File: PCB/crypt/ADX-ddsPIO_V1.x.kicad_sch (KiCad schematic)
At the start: 74 parts, among them J1 Conn_Coaxial, J2 +12V, Q1 BS170, Q2 BS170, Q3 BS170, Q5 BS170, U1 L7805, U2 74LS244, U4 CD2003GB_GP

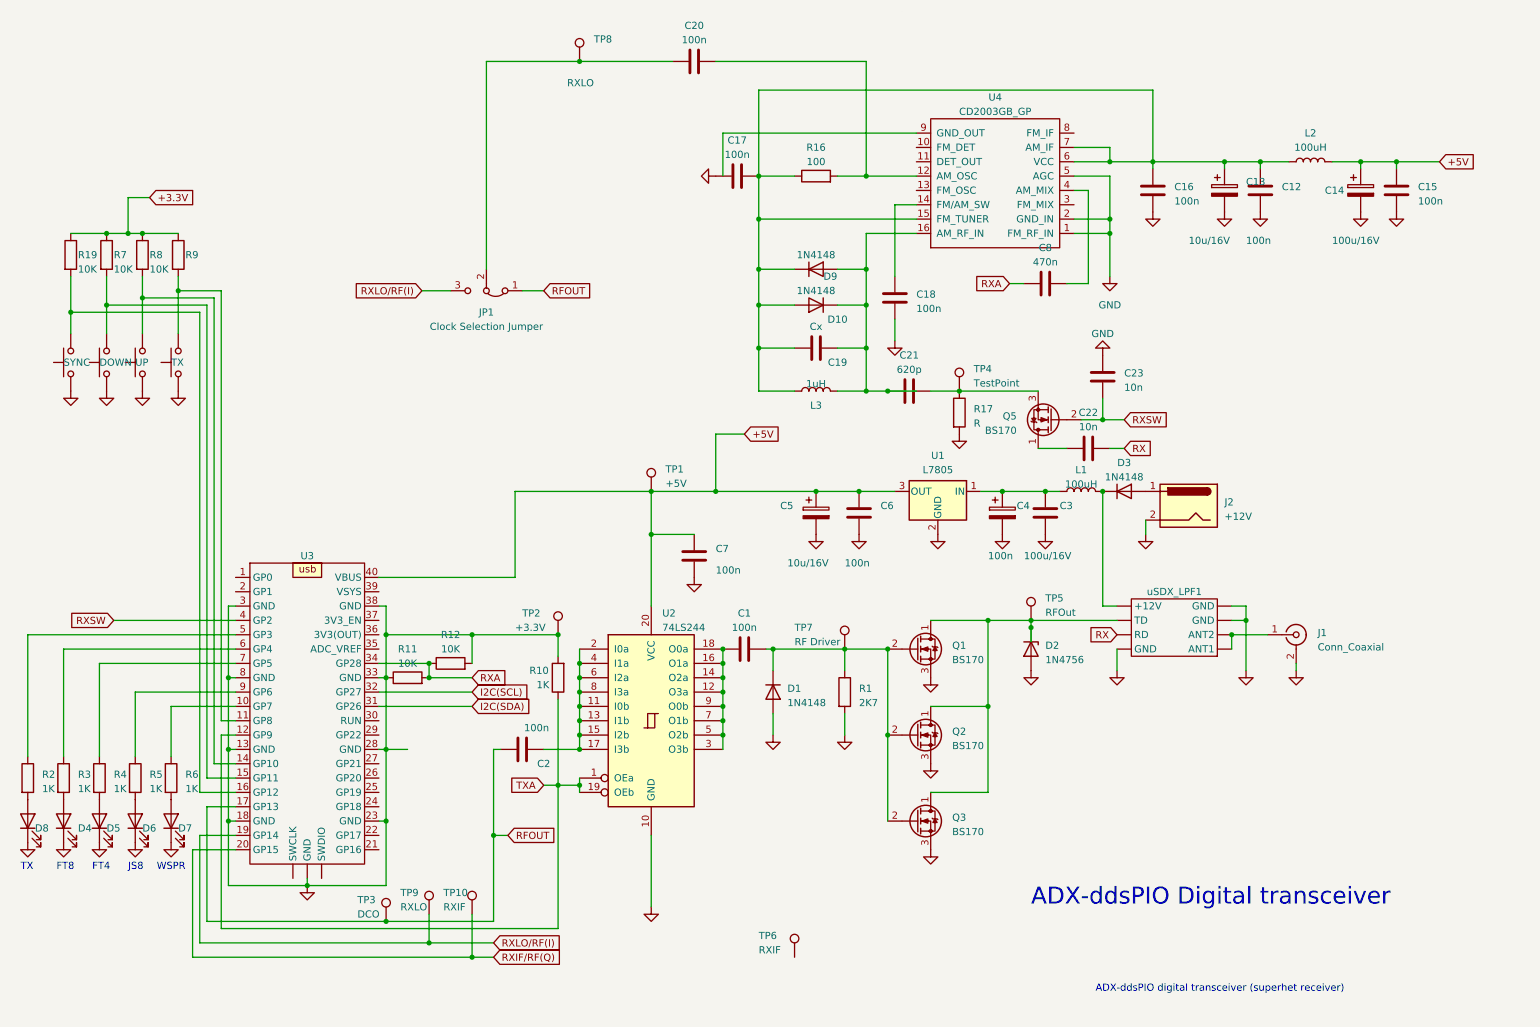
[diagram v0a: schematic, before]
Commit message: wiring
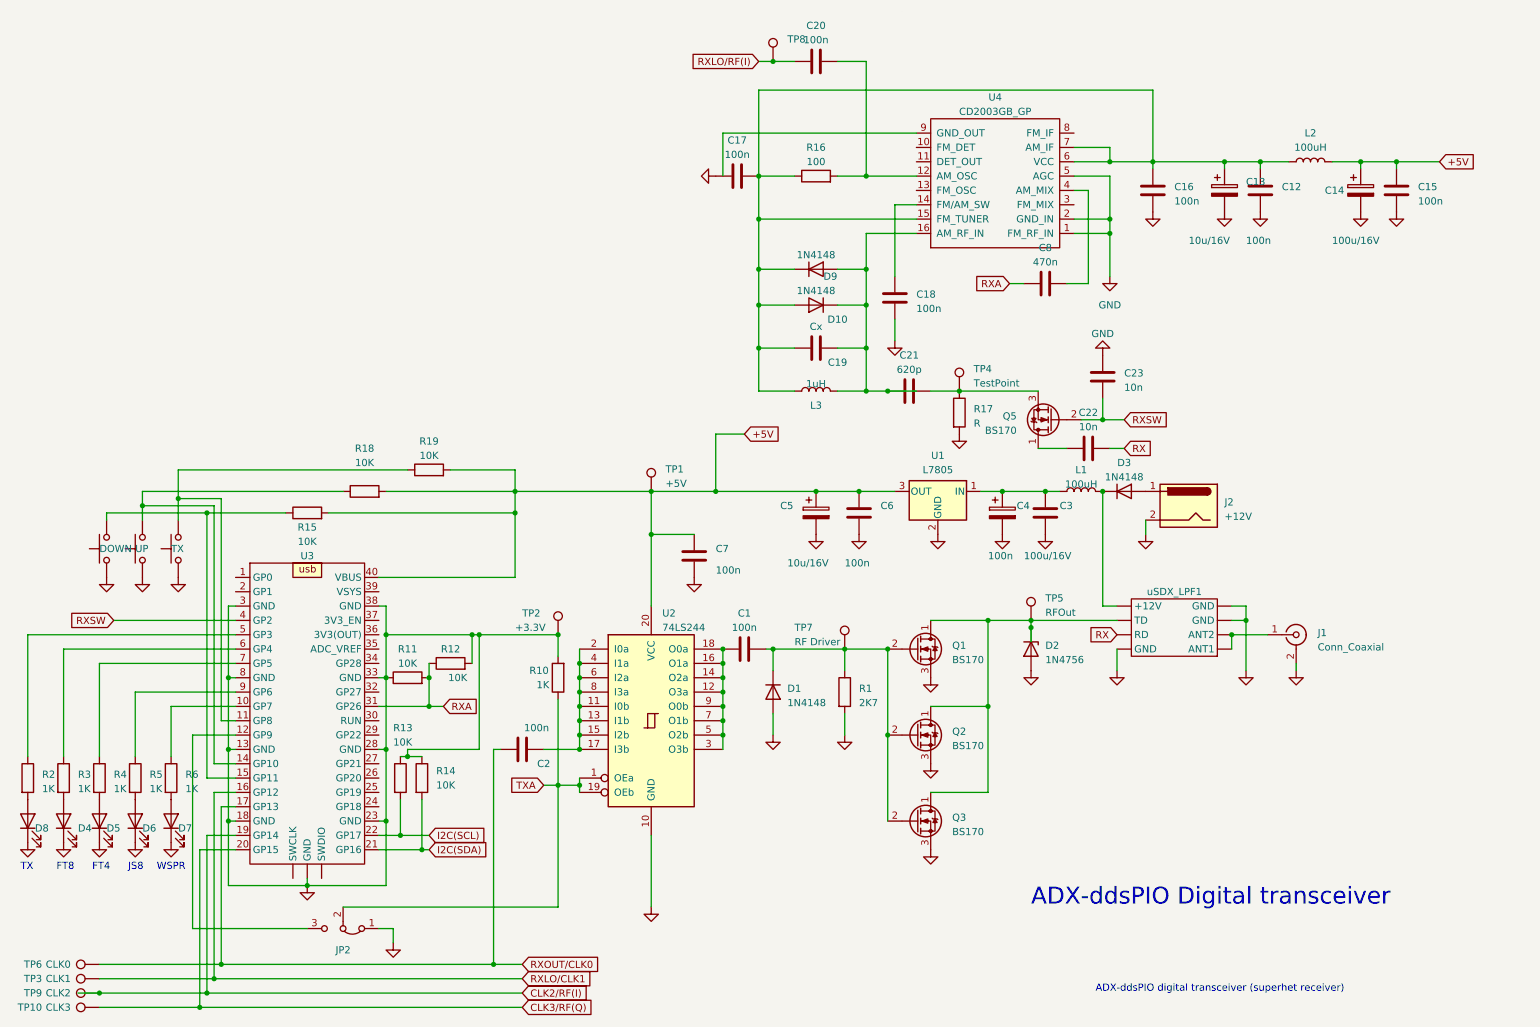
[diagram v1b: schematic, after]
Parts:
- removed JP1: Clock Selection Jumper, symbol Jumper:Jumper_3_Bridged12
- removed R7, R8, R9: 10K, symbol Device:R
- removed SYNC: SW_MEC_5G, symbol Switch:SW_MEC_5G
- added JP2: ~, symbol Jumper:Jumper_3_Bridged12
- added R13, R14, R15, R18: 10K, symbol Device:R
- TP10: value RXIF -> CLK3
- TP3: value DCO -> CLK1
- TP6: value RXIF -> CLK0
- TP9: value RXLO -> CLK2
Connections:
- net +3.3V is gone; now on an unnamed net: R19.1
- net +5V: now also R19.2, R15.2, R18.2
- net GND: now also JP2.1 (A), R13.1, R14.1
- net I2C(SCL): now also U3.22 (GP17), R13.2; no longer U3.32 (GP27)
- net I2C(SDA): now also U3.21 (GP16), R14.2; no longer U3.31 (GP26)
- net RXA: now also U3.31 (GP26); no longer U3.34 (GP28)
- net RXLO/RF(I): now also C20.1, TP8.1; no longer TP9.1, U3.19 (GP14)
- net TXA: now also JP2.2 (C); no longer U3.12 (GP9)
- net RXOUT/CLK0: now reaches TP6.1
- net RXOUT/CLK0: now also C2.1, U3.17 (GP13)
- net RXLO/CLK1: now reaches U3.16 (GP12)
- net RXLO/CLK1: now also TP3.1; no longer R19.2
- net at U3.14 (GP10), UP.3 (B), UP.4 (B): now also R18.1
- net at DOWN.3 (B), DOWN.4 (B), U3.15 (GP11): now also R15.1
- removed net RFOUT: C2.1, TP3.1, U3.17 (GP13)
- net RXIF/RF(Q) renamed CLK3/RF(Q)
- new net: JP2.3 (B), U3.12 (GP9)
- new net CLK2/RF(I): TP9.1, U3.19 (GP14)
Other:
- moved on the sheet: C20, DOWN, TP6, TP8, TX, UP
